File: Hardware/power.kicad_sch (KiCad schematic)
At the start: 44 parts, among them J3 XT30, J5 Conn_01x02, J6 Conn_01x02, J7 SERVO_CONN_01, J8 SERVO_CONN_02, J9 SERVO_CONN_02, Q1 FDN340P, Q2 DMP3013SFV, Q3 CSD17577Q3A, Q4 CSD17577Q3A, U10 LTC4412, U11 UCC27517A, U12 UCC27517A, U6 MP2331, U7 KA78M05, U9 LTC4412

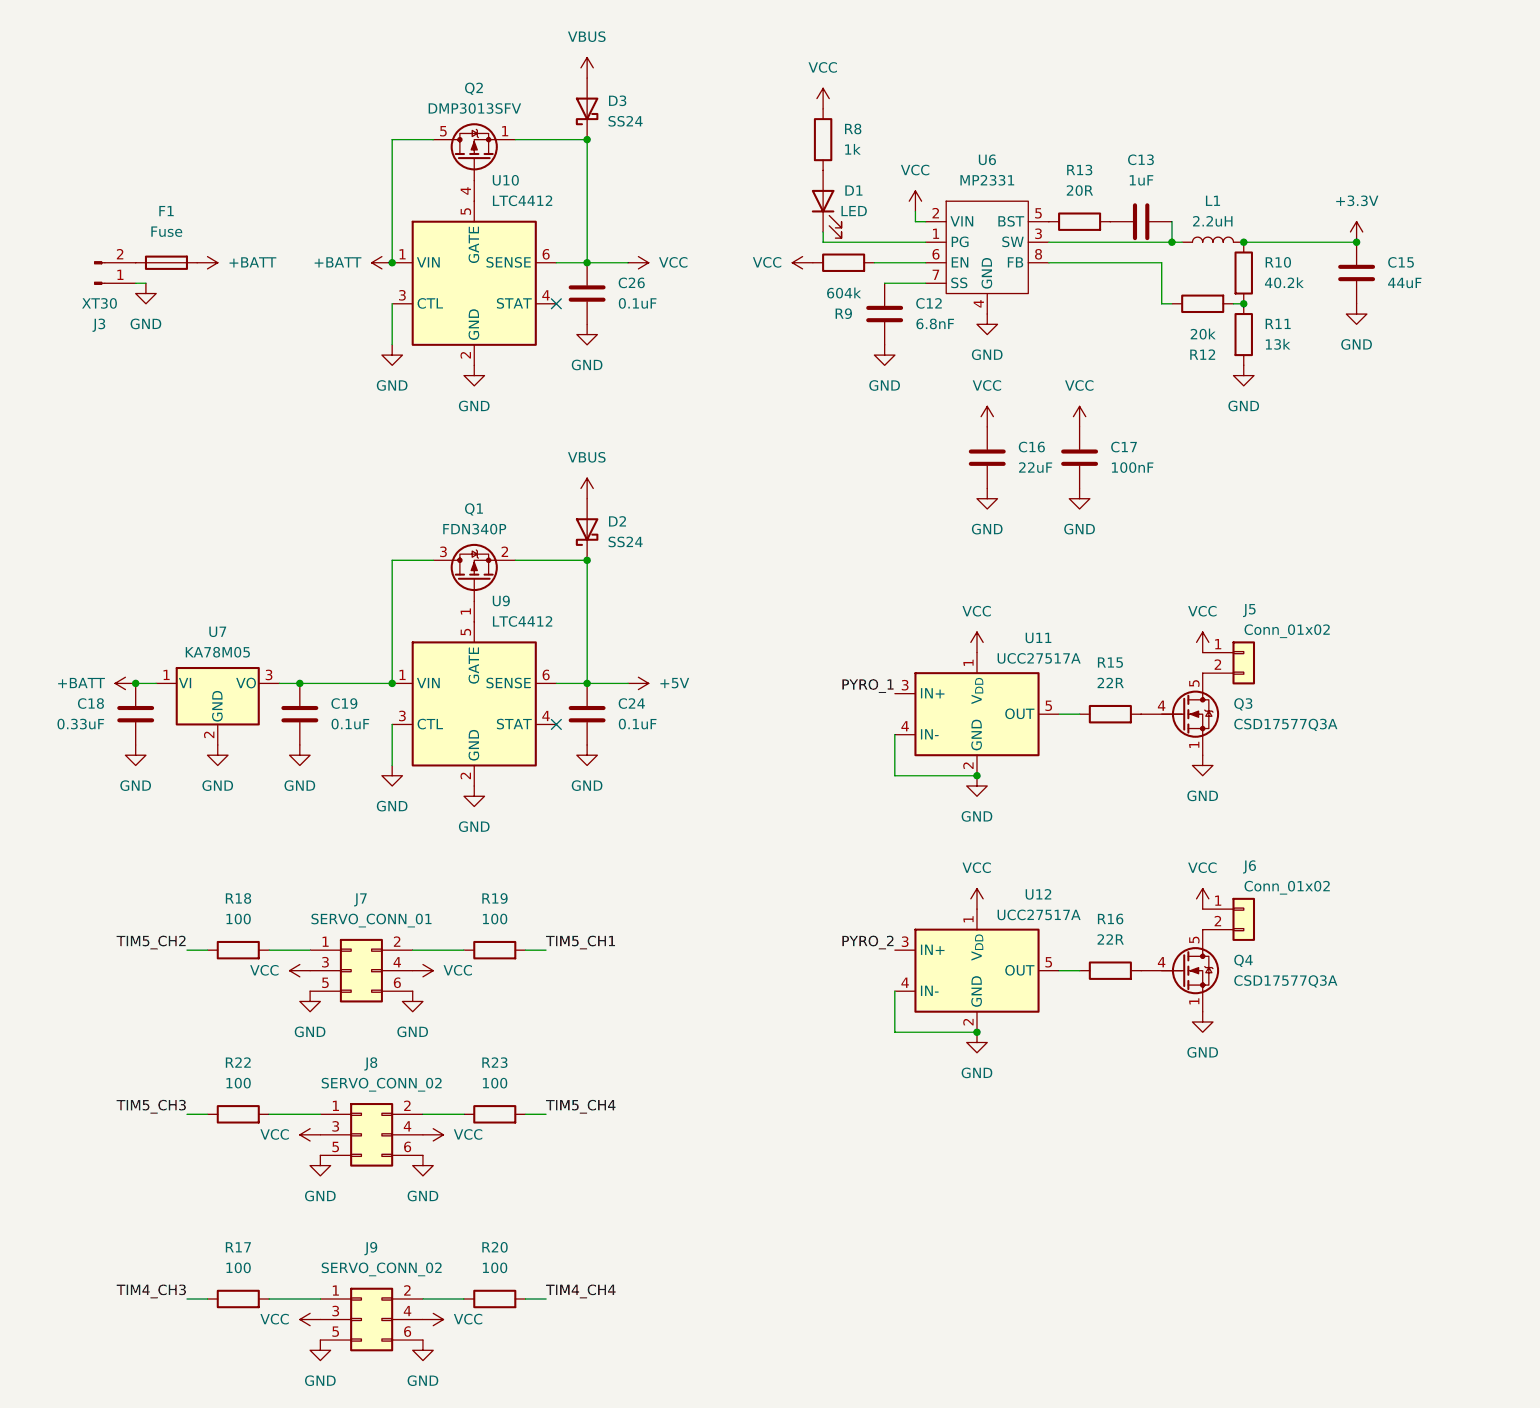
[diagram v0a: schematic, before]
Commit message: Minor changes in sensors and peripherals
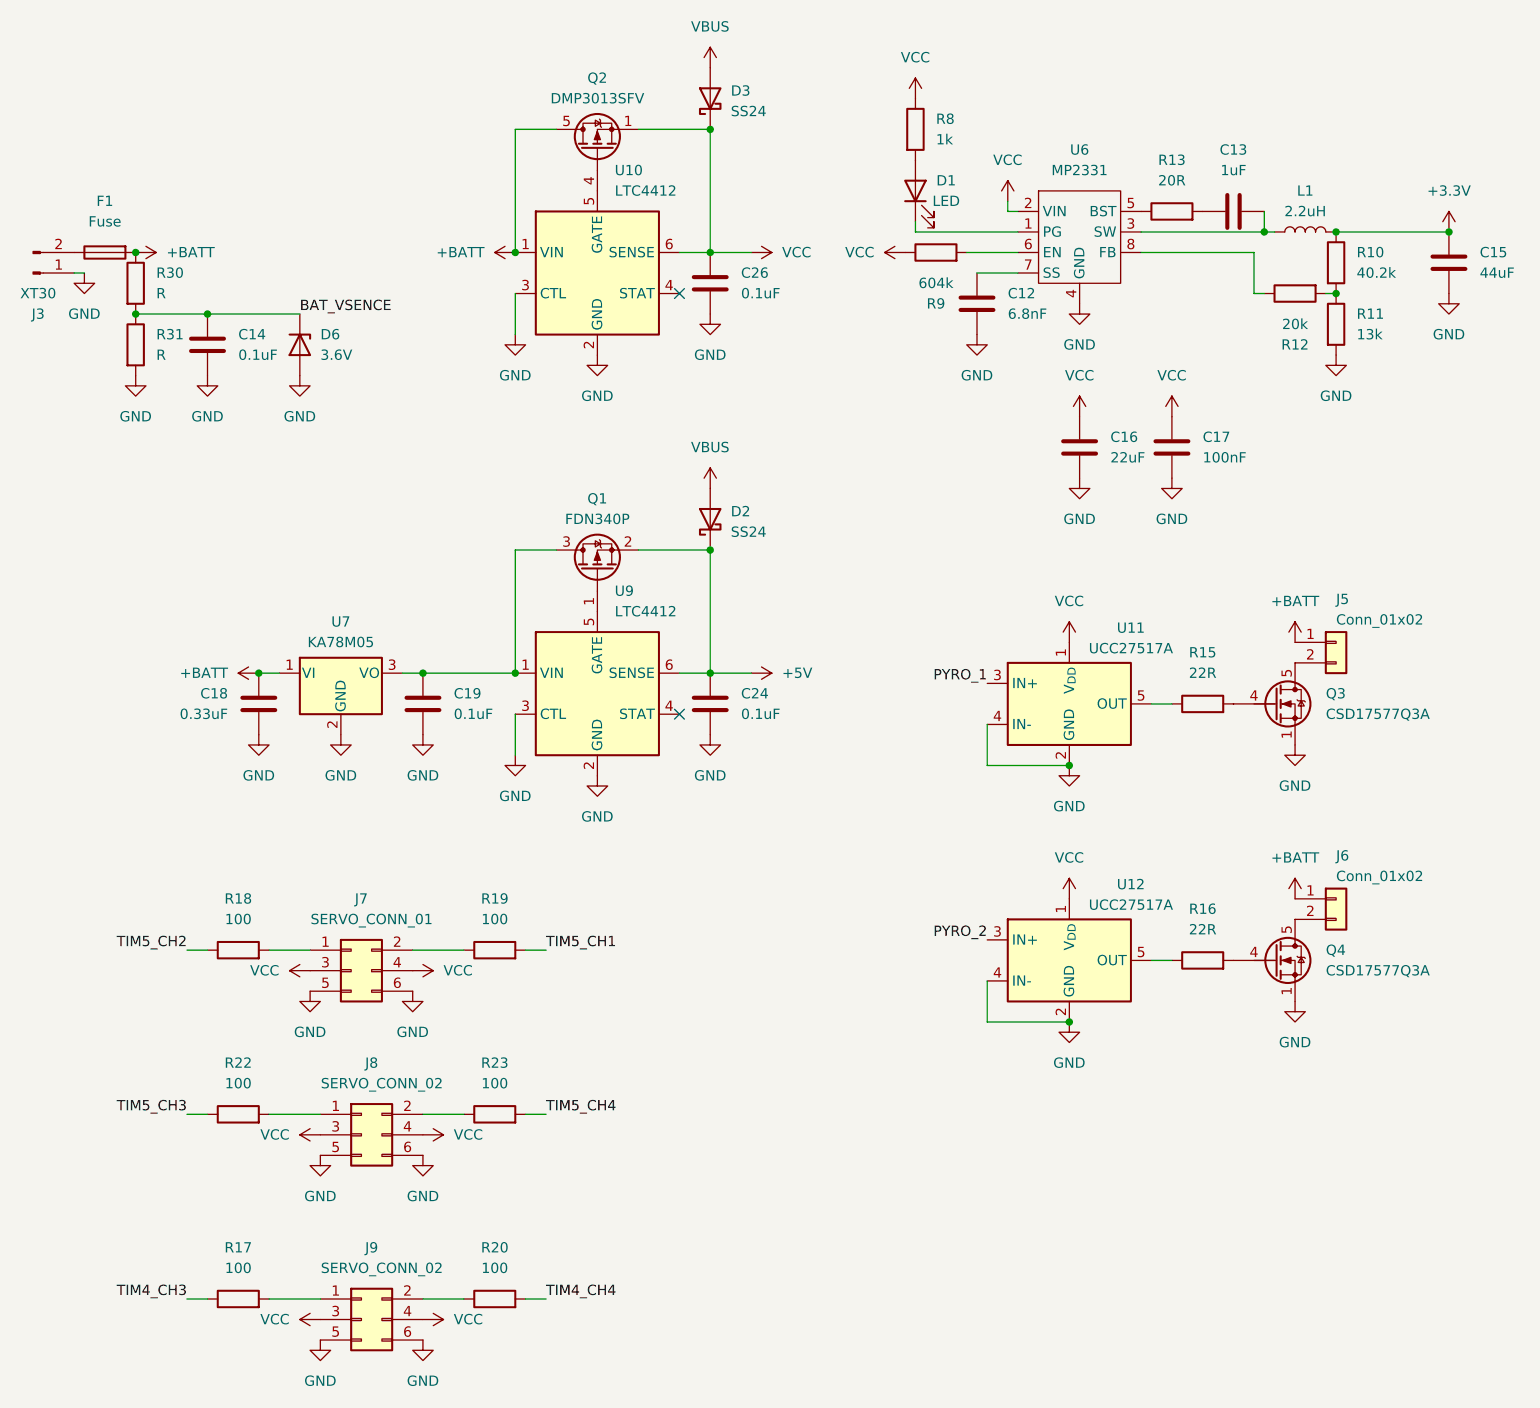
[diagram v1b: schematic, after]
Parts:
- added C14: 0.1uF, symbol Device:C
- added D6: 3.6V, symbol Device:D_Zener
- added R30, R31: R, symbol Device:R
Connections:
- net +BATT: now also J5.1 (Pin_1), J6.1 (Pin_1), R30.1
- net GND: now also C14.2, D6.2 (A), R31.2
- net VCC: no longer J5.1 (Pin_1), J6.1 (Pin_1)
- new net BAT_VSENCE: C14.1, D6.1 (K), R30.2, R31.1
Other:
- moved on the sheet: C12, C13, C15, C16, C17, C18, C19, C24, C26, D1, D2, D3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
